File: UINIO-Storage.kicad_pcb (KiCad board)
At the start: 2 copper layers, 60 x 42 mm, 55 parts, among them J1 Conn_01x04_Pin, J2 Conn_01x04_Pin, J3 Conn_01x06_Pin, J4 Conn_01x08_Pin, J5 Conn_01x06_Pin, U1 I2C-24-EEPROM-SOIC8, U2 I2C-24-EEPROM-TSSOP8, U3 SPI-25-Flash-SOIC8, U4 ME6211, U5 SPI-25-Flash-WSON8

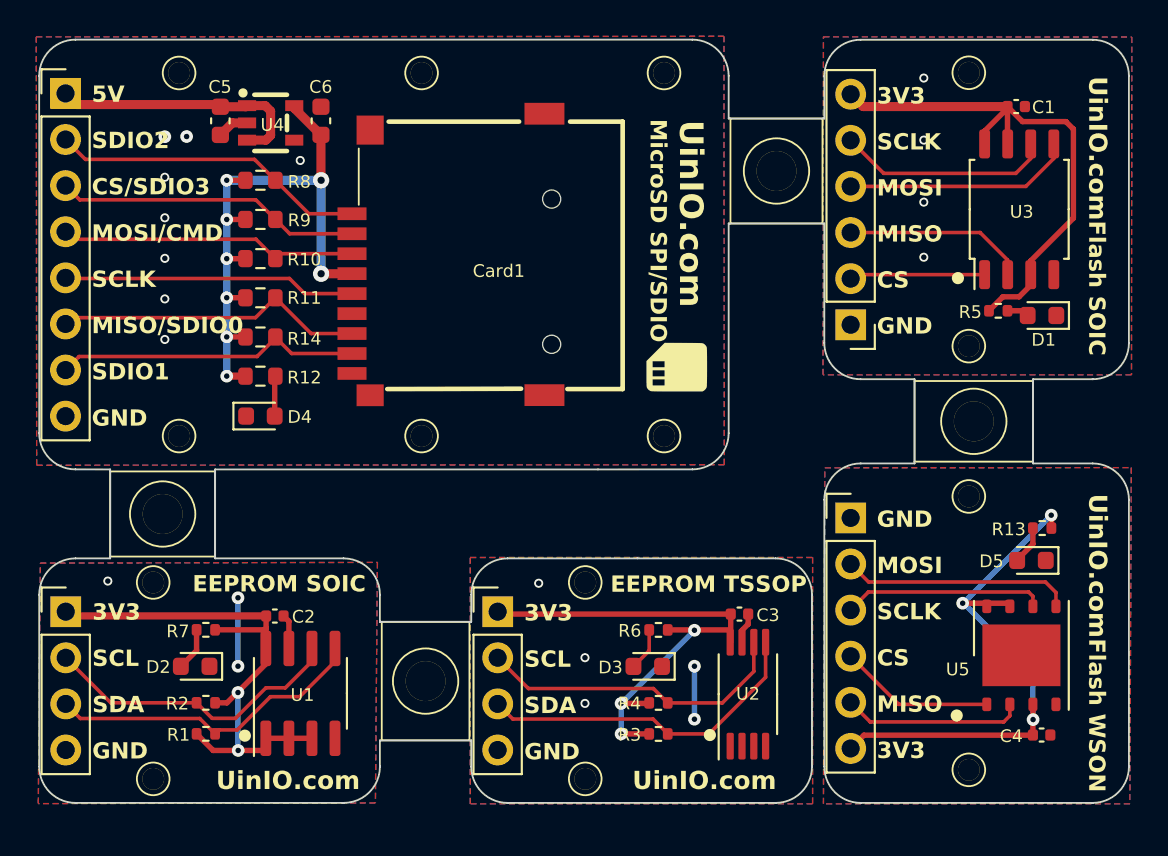
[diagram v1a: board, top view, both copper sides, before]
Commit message: Release UINIO-Storage version 1.0.0.
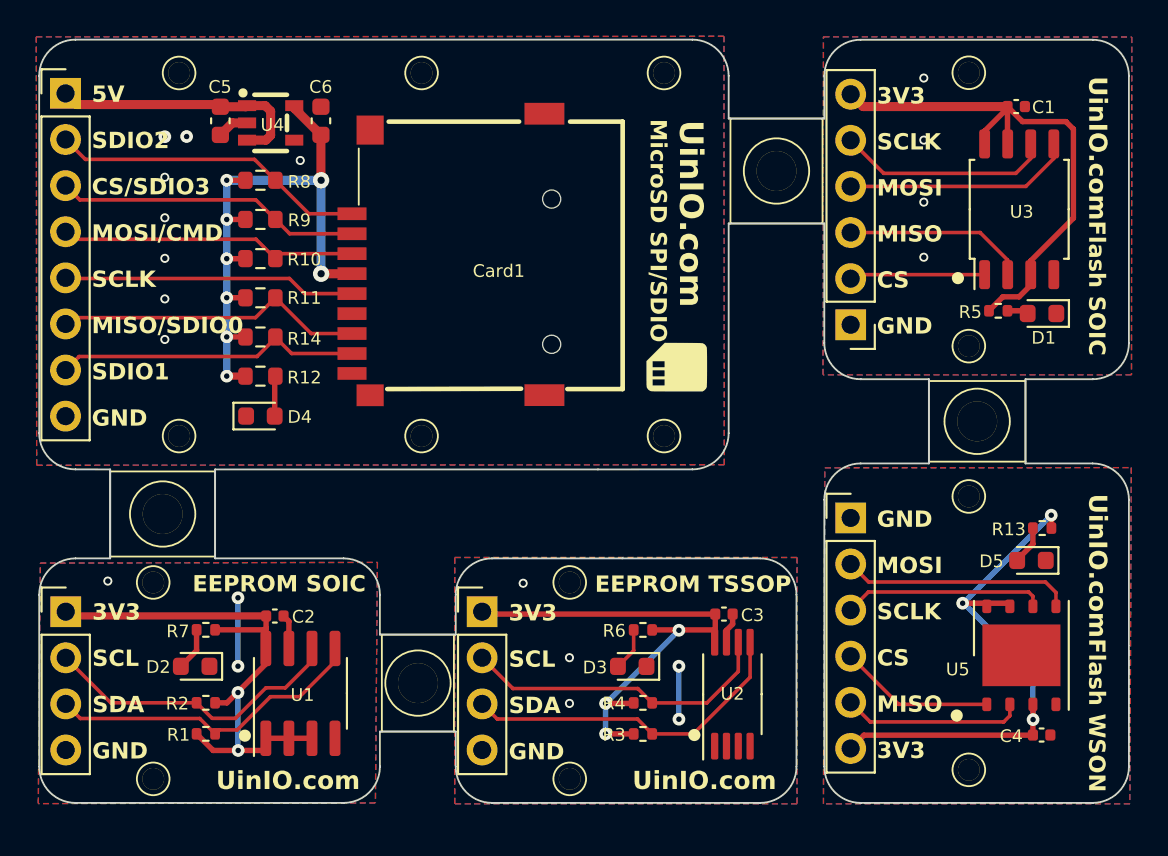
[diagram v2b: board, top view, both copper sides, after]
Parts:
- moved J2 0.86 mm to (146.0, 114.7)
- moved U2 0.86 mm to (159.8, 119.2)
- moved C3 0.85 mm to (159.3, 114.8)
- moved D3 0.85 mm to (154.2, 117.7)
- moved HOLE** 0.85 mm to (150.8, 123.9)
- moved HOLE** 0.85 mm to (150.8, 113.1)
- moved R3 0.85 mm to (154.8, 121.4)
- moved R4 0.85 mm to (154.8, 119.7)
- moved R6 0.85 mm to (154.8, 115.7)
- moved HOLE** 0.43 mm to (142.4, 118.6)
- moved HOLE** 0.19 mm to (173.2, 104.2)
- moved D1 0.11 mm to (176.8, 98.2)
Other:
- outline, holes or cut-outs redrawn
